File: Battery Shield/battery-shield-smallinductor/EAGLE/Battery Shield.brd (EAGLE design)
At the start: 58.5 x 15.2 mm, 32 parts, among them IC1 MCP73871, U1 TPS61200

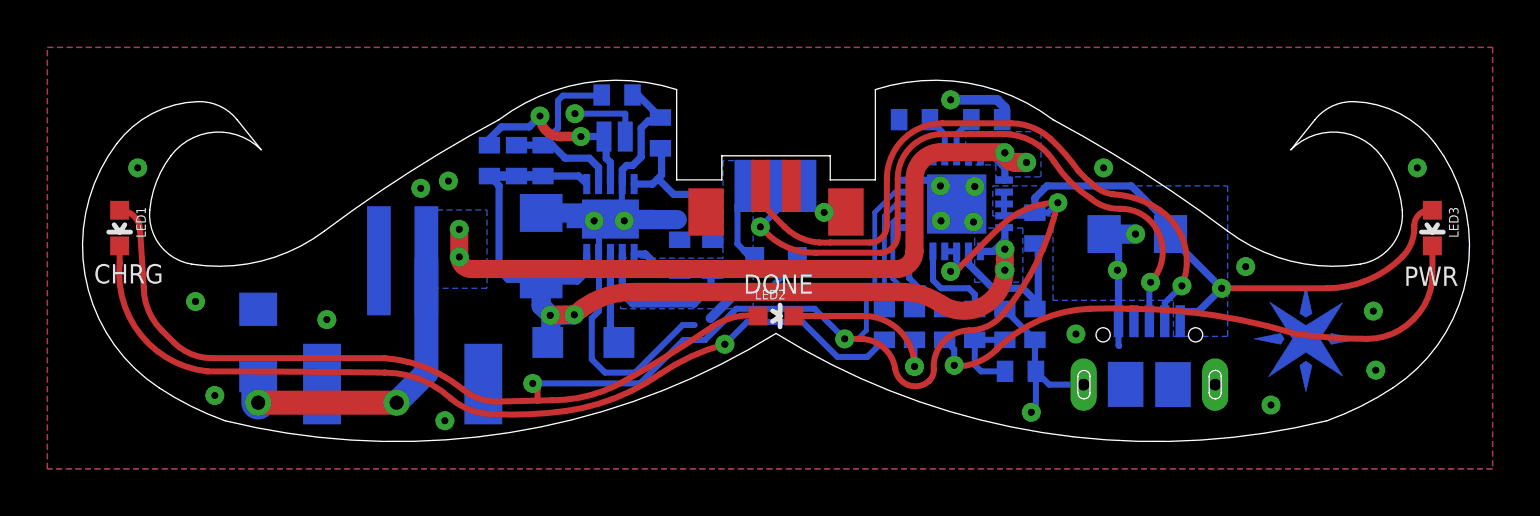
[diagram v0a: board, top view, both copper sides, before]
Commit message: updated battery shield gerbers to v201
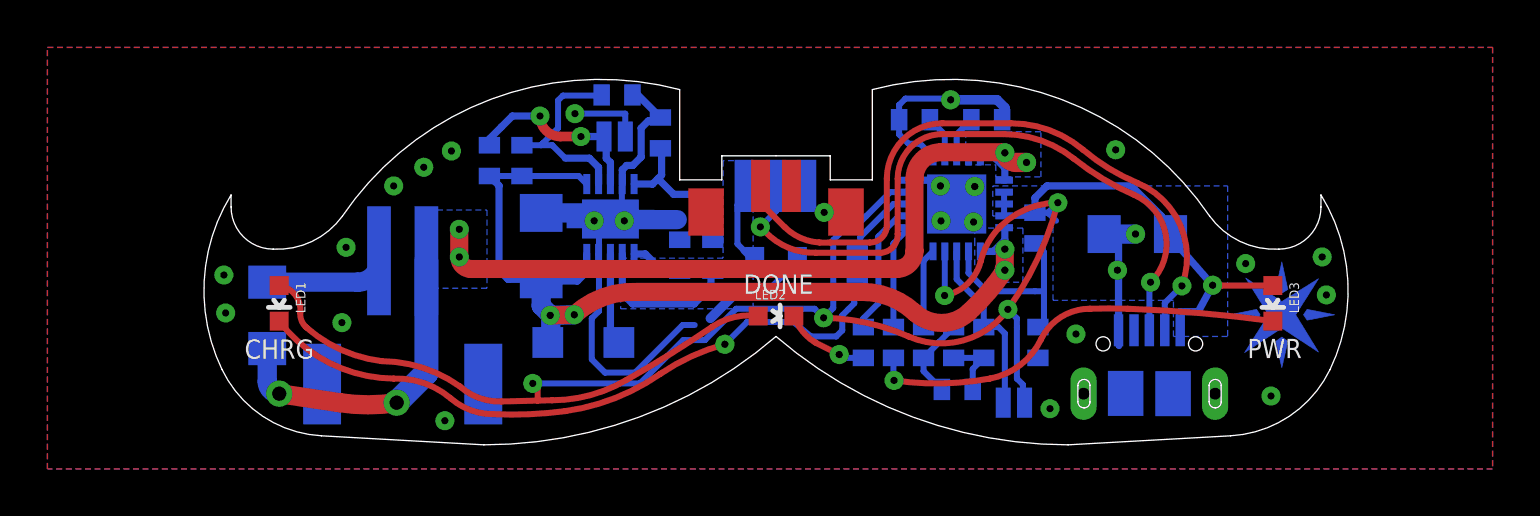
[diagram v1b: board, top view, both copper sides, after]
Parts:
- removed C2: 0.1uF, SparkFun-Passives:0402-CAP
- added R14: 10K, SparkFun-Passives:0402-RES
- added SJ2: SOLDERJUMPERNO, SparkFun-Passives:SJ_2S-NO
- moved LED1 7.44 mm to (25.0, 5.71)
- moved LED3 7.44 mm to (66.9, 5.71)
- moved R6 2.77 mm to (53.6, 2.08)
- moved R11 2.67 mm to (49.4, 7.24)
- moved R12 2.29 mm to (49.7, 4.06)
- moved R13 2.29 mm to (50.9, 4.06)
- moved RT1 2.29 mm to (52.2, 4.06)
- moved RT2 2.29 mm to (53.5, 4.06), turned to 90 degrees
- moved U$2 1.44 mm to (67.3, 5.23)
- moved C3 1.20 mm to (24.5, 5.21)
- moved R3 0.89 mm to (35.3, 11.7)
- moved R10 0.77 mm to (57.0, 4.06)
- moved JP1 0.38 mm to (61.7, 1.91)
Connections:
- new net N$20: IC1.3, R14.2, SJ2.2
- net GND: now also R14.1
- net N$3: no longer C2.2
- net VBATT_OUT: no longer C2.1
- net VBUS: now also SJ2.1; no longer IC1.3
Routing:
- net VBUS: track 104.4 -> 90.4 mm, vias 5 -> 6
- net N$8: track 37.4 -> 28.2 mm
- net N$20: track 0.00 -> 7.62 mm
- net N$16: track 24.7 -> 17.9 mm
- net GND: track 45.3 -> 51.4 mm
- net N$10: track 7.10 -> 3.72 mm
- net N$6: track 5.18 -> 3.32 mm
- net N$12: track 7.30 -> 8.35 mm
- net N$14: track 4.85 -> 5.75 mm
- net VBATT_OUT: track 40.1 -> 40.7 mm
- net N$9: track 3.87 -> 3.36 mm
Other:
- board size 58.5 x 15.2 mm -> 48.3 x 15.4 mm
- board text added: "Battery Shield v2.0.1"
- board text added: "J1"
- board text added: "J2"
- board text added: "spark.io"
- board text removed: "Battery Shield"
